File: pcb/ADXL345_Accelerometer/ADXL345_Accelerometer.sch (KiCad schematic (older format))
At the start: 16 parts, among them J1 Conn_01x09, Q1 BSS138, Q2 BSS138, U1 ADXL345_Library, U2 AP2112K-3.3

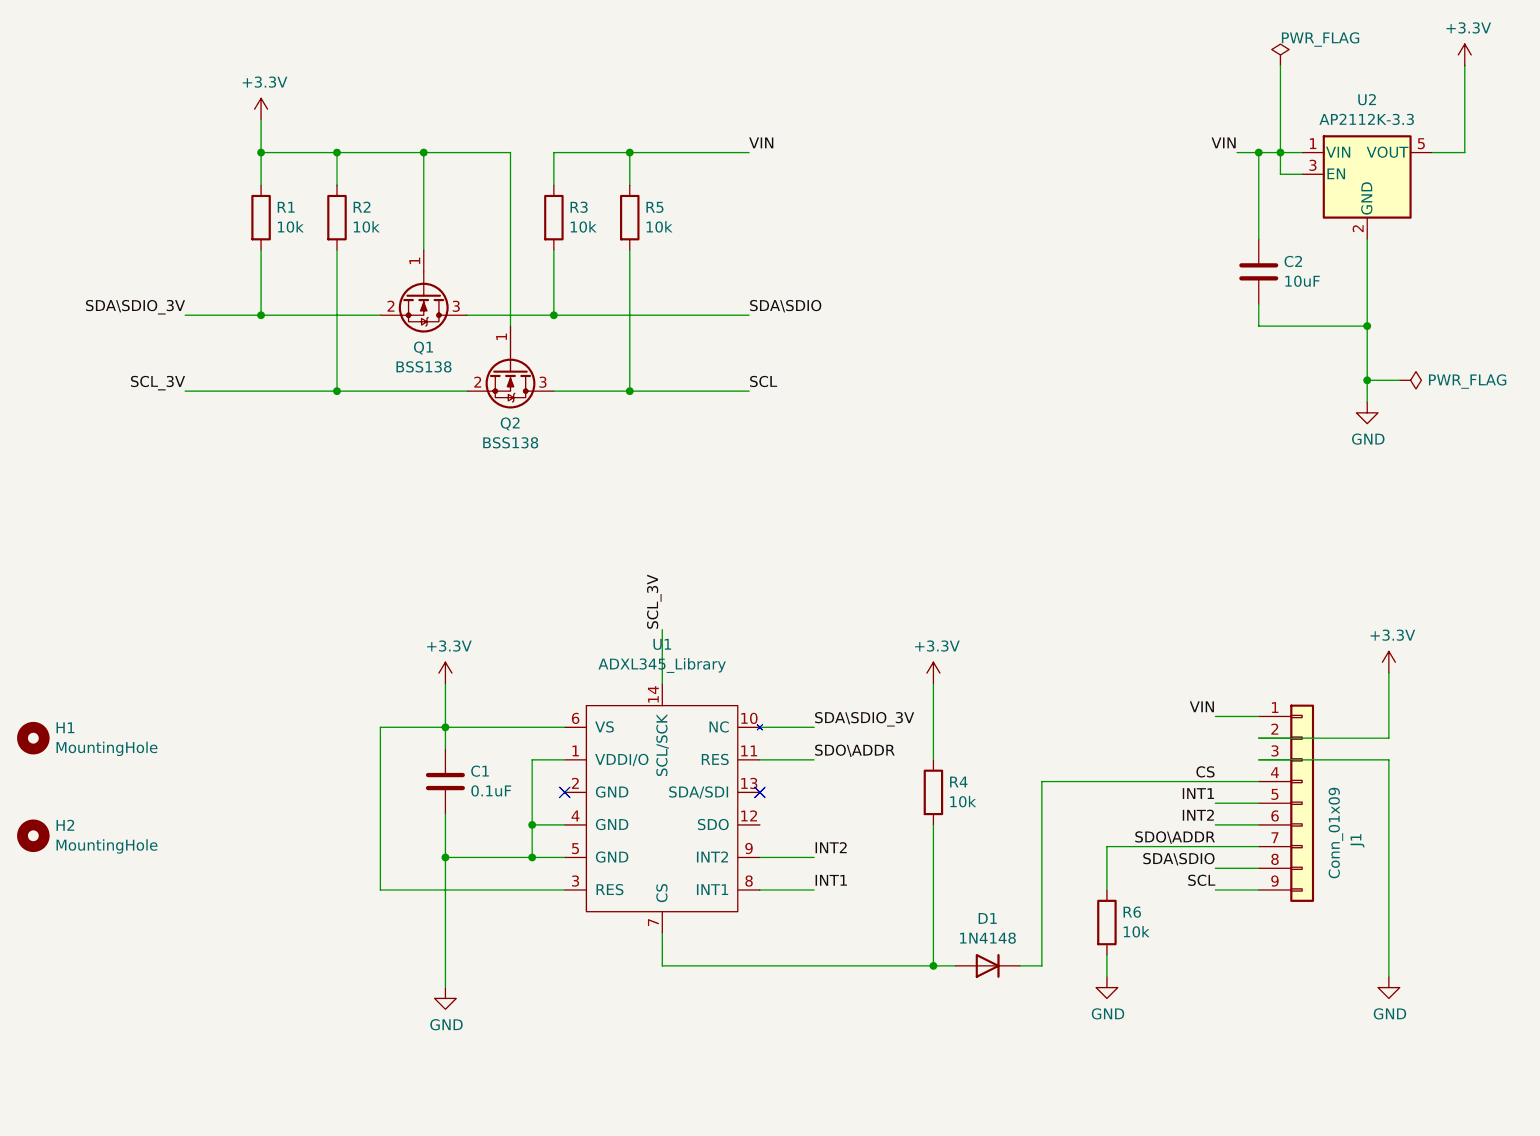
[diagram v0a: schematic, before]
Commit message: Correcciones
Se corrigieron segun las recomendaciones realizadas por el docente.
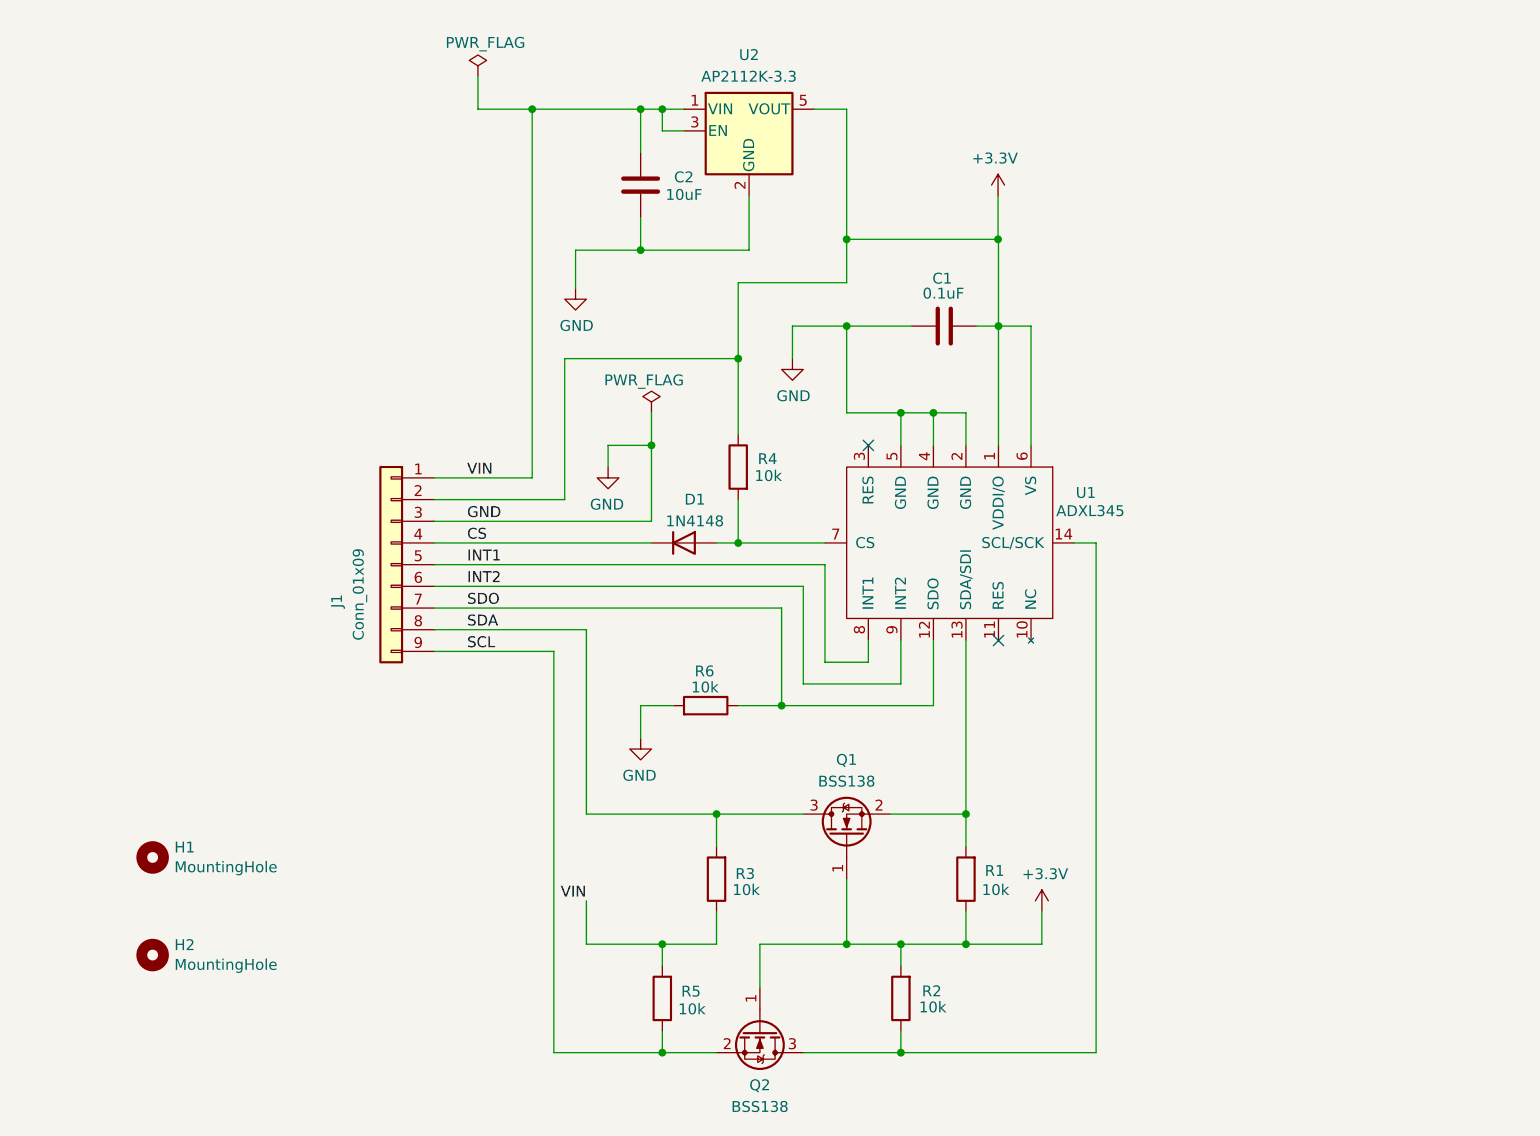
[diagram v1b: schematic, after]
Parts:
- U1: value ADXL345_Library -> ADXL345
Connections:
- net +3V3: now also R2.2, U1.1 (VDDI/O); no longer R2.1, U1.3 (RES)
- net GND: now also U1.2 (GND); no longer U1.1 (VDDI/O)
- net SCL: now also Q2.2 (S), R5.1; no longer Q2.3 (D), R5.2
- net VIN: now also R5.2; no longer R5.1
- net SDO: now reaches U1.12 (SDO)
- net SDO: now also J1.7 (Pin_7), R6.1
- net at U1.13 (SDA/SDI): now also Q1.2 (S), R1.2
- removed net SCL_3V: Q2.2 (S), R2.2, U1.14 (SCL/SCK)
- net SDA\SDIO renamed SDA
- removed net SDA\SDIO_3V: Q1.2 (S), R1.2, U1.10 (NC)
- removed net SDO\ADDR: J1.7 (Pin_7), R6.1, U1.11 (RES)
- new net: Q2.3 (D), R2.1, U1.14 (SCL/SCK)
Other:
- moved on the sheet: C1, C2, D1, H1, H2, J1, Q1, Q2, R1, R2, R3, R4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
